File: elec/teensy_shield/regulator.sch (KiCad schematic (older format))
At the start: 1 part

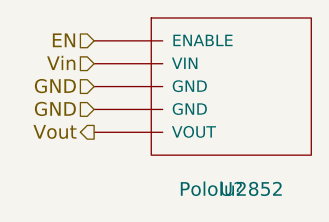
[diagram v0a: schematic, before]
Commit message: Elec ?
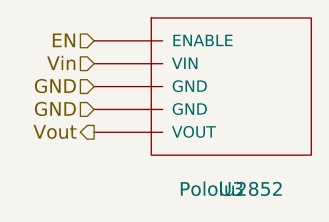
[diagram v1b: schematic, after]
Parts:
- gave numbers to parts that had none: 1
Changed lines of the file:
@@
 EN
 $Comp
-L Pololu2852 U?
+L Pololu2852 U12
 U 1 1 55E8368A
 P 5850 3900
-F 0 "U?" H 5800 3500 60  0000 C CNN
+AR Path="/55E6307C/55E63161/55E8368A" Ref="U12"  Part="1"
+AR Path="/55E7381B/55E63161/55E8368A" Ref="U3"  Part="1"
+AR Path="/55E7381C/55E63161/55E8368A" Ref="U6"  Part="1"
+AR Path="/55E7381D/55E63161/55E8368A" Ref="U9"  Part="1"
+F 0 "U3" H 5800 3500 60  0000 C CNN
 F 1 "Pololu2852" H 5800 3500 60  0000 C CNN
 F 2 "" H 5800 3500 60  0000 C CNN
